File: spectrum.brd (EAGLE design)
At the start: 100 x 31.1 mm, 40 parts, among them CN1 PH-1X06RG, CN2 PH-1X04SG, CN3 PH-1X04SG, CN4 FH-1X06RG, CN5 PH-1X04SGRG, CN6 FH-1X04RG, IC1 7W14FU, IC2 7W14FU, IC3 7W14FU, IC5 NJM2670E3, IC6 NJM2670E3, IC7 NJM2670E3, IC8 R5F104BCAFP, Q1 BSS84, Q2 BSS84

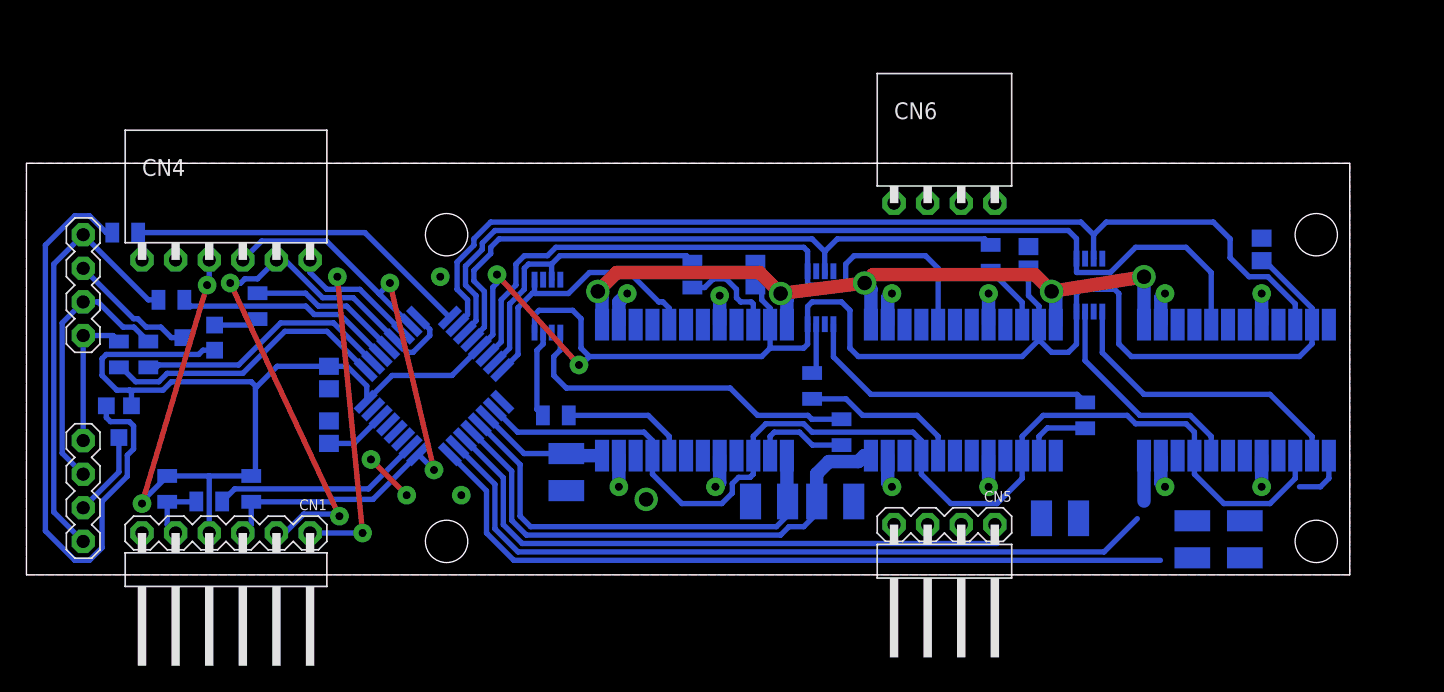
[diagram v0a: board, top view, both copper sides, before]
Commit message: Complete routing for the first time
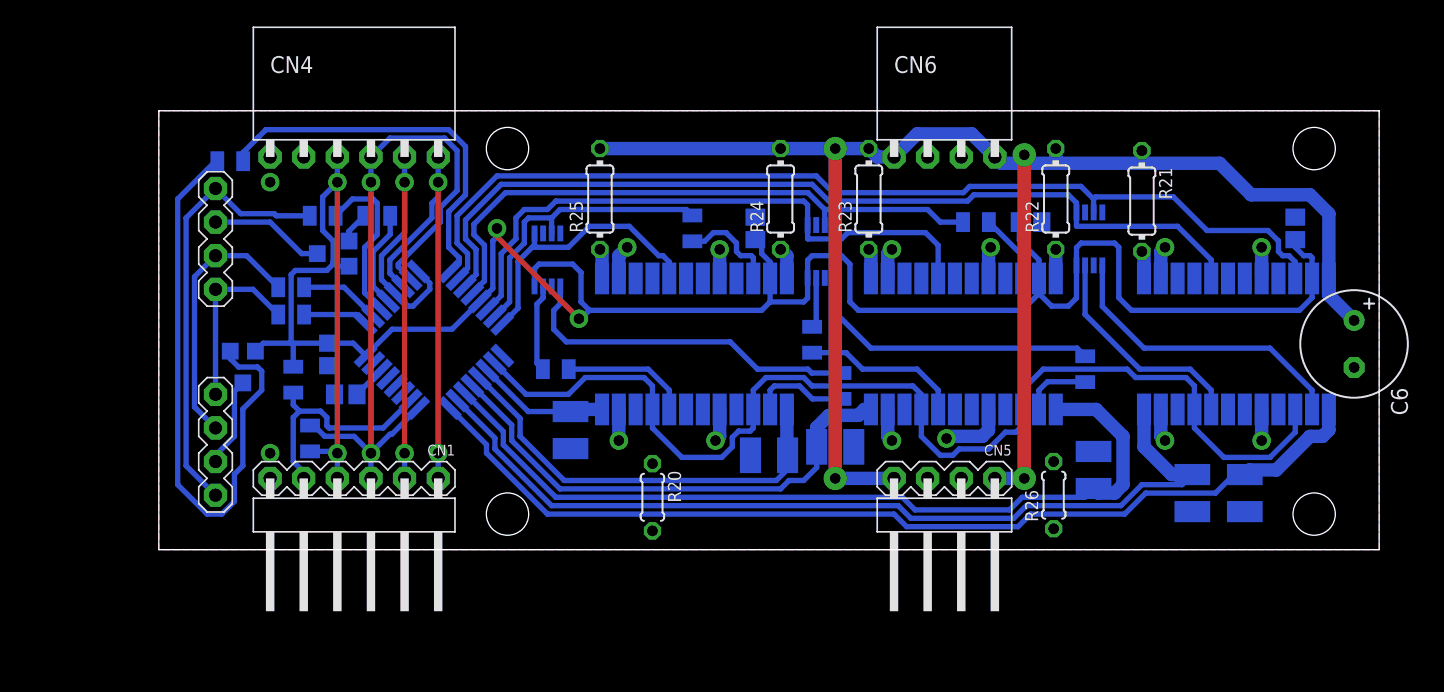
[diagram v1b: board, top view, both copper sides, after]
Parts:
- added C6: 1500u, MyLib:E3,5-8
- added R21, R22, R23, R24, R25: 0, MyLib:0204/7
- added R26: 0, MyLib:0204/5
- R20: device MyLib:R2012 -> MyLib:0204/5
- moved R20 33.5 mm to (47.3, 5.87), flipped to the top, turned to 270 degrees
- moved R19 13.4 mm to (20.0, 19.7), turned to 0 degrees
- moved R17 13.1 mm to (22.4, 27.1)
- moved R8 12.6 mm to (20.2, 14.8)
- moved CN4 12.4 mm to (24.8, 31.6)
- moved Q2 12.0 mm to (23.2, 24.3)
- moved R18 11.9 mm to (20.0, 21.7), turned to 0 degrees
- moved R15 11.3 mm to (26.5, 27.1), turned to 0 degrees
- moved CN2 10.6 mm to (14.3, 25.4)
- moved CN3 10.6 mm to (14.3, 9.84)
- moved CN1 10.5 mm to (24.8, 7.30)
- moved Q1 10.2 mm to (16.4, 15.7)
- moved R16 9.60 mm to (15.4, 31.3)
- moved R7 5.85 mm to (21.4, 10.3), turned to 90 degrees
- moved CN5 5.40 mm to (69.4, 7.30)
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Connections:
- removed net N$44: IC8.2, R20.2
- new net N$47: IC7.13, R25.1
- net GND: now also C6.-, CN5.2, CN5.3, CN6.2, CN6.3, R20.1, R20.2, R26.1, R26.2
- net N$13: now also C6.+, CN5.1, CN5.4, CN6.1, CN6.4, R21.1, R22.2, R23.2, R24.2, R25.2; no longer IC5.13, IC6.13, IC6.24, IC7.13, IC7.24
- net N$42: now also IC5.13, R21.2; no longer CN5.3, CN6.2
- net N$43: now also IC6.24, R22.1; no longer CN5.2, CN6.3
- net N$45: now also IC6.13, R23.1; no longer CN5.1, CN6.4
- net N$46: now also IC7.24, R24.1; no longer CN5.4, CN6.1
- net RESET: now also IC8.2; no longer R20.1
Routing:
- net N$13: track 58.5 -> 126.2 mm, vias 5 -> 4
- net +5V: track 199.4 -> 177.0 mm
- net N$5: track 45.6 -> 64.6 mm
- net N$41: track 22.0 -> 4.95 mm
- net N$44: track 16.0 -> 0.00 mm
- net N$40: track 19.6 -> 6.13 mm
- net RESET: track 4.83 -> 17.4 mm
- net N$1: track 63.1 -> 75.1 mm
- net N$2: track 61.1 -> 68.4 mm
- net N$19: track 45.8 -> 39.1 mm
- net TOOL0: track 50.0 -> 54.2 mm
- net N$36: track 11.6 -> 7.48 mm
- net N$32: track 16.6 -> 12.7 mm
- net GND: track 3.82 -> 0.00 mm, vias 5 -> 2
- net N$4: track 71.8 -> 68.4 mm
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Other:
- board size 100 x 31.1 mm -> 92.2 x 33.2 mm
